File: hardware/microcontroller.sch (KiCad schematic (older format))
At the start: 30 parts, among them P1 USB_OTG, P2 ICSP, P3 JTAG, SW1 Reset, U1 ATMEGA32U4-AU, X1 16MHz

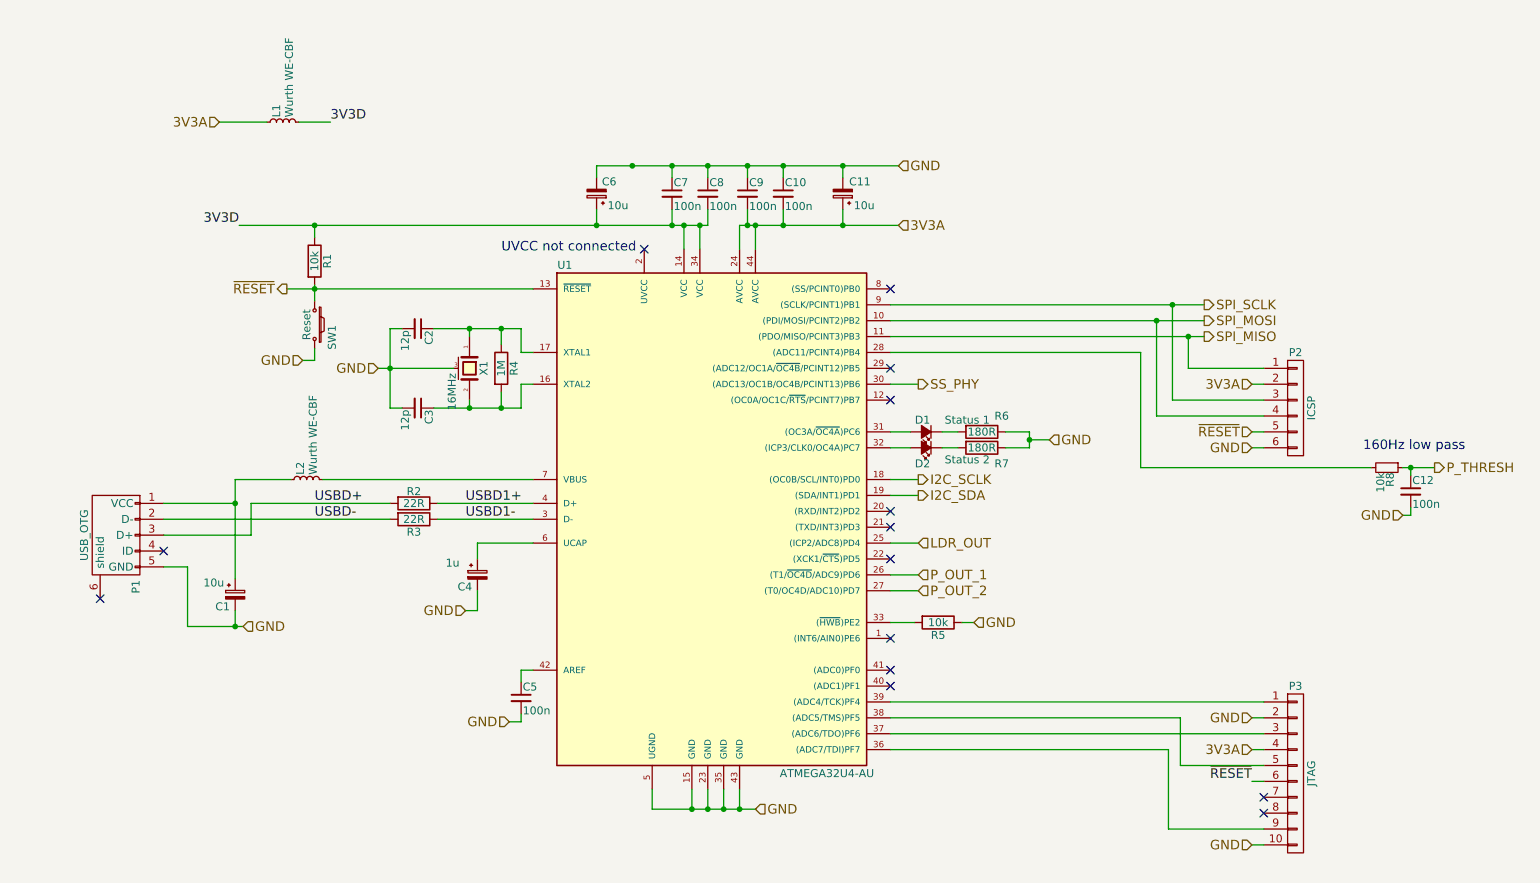
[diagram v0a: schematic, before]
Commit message: New revision to board
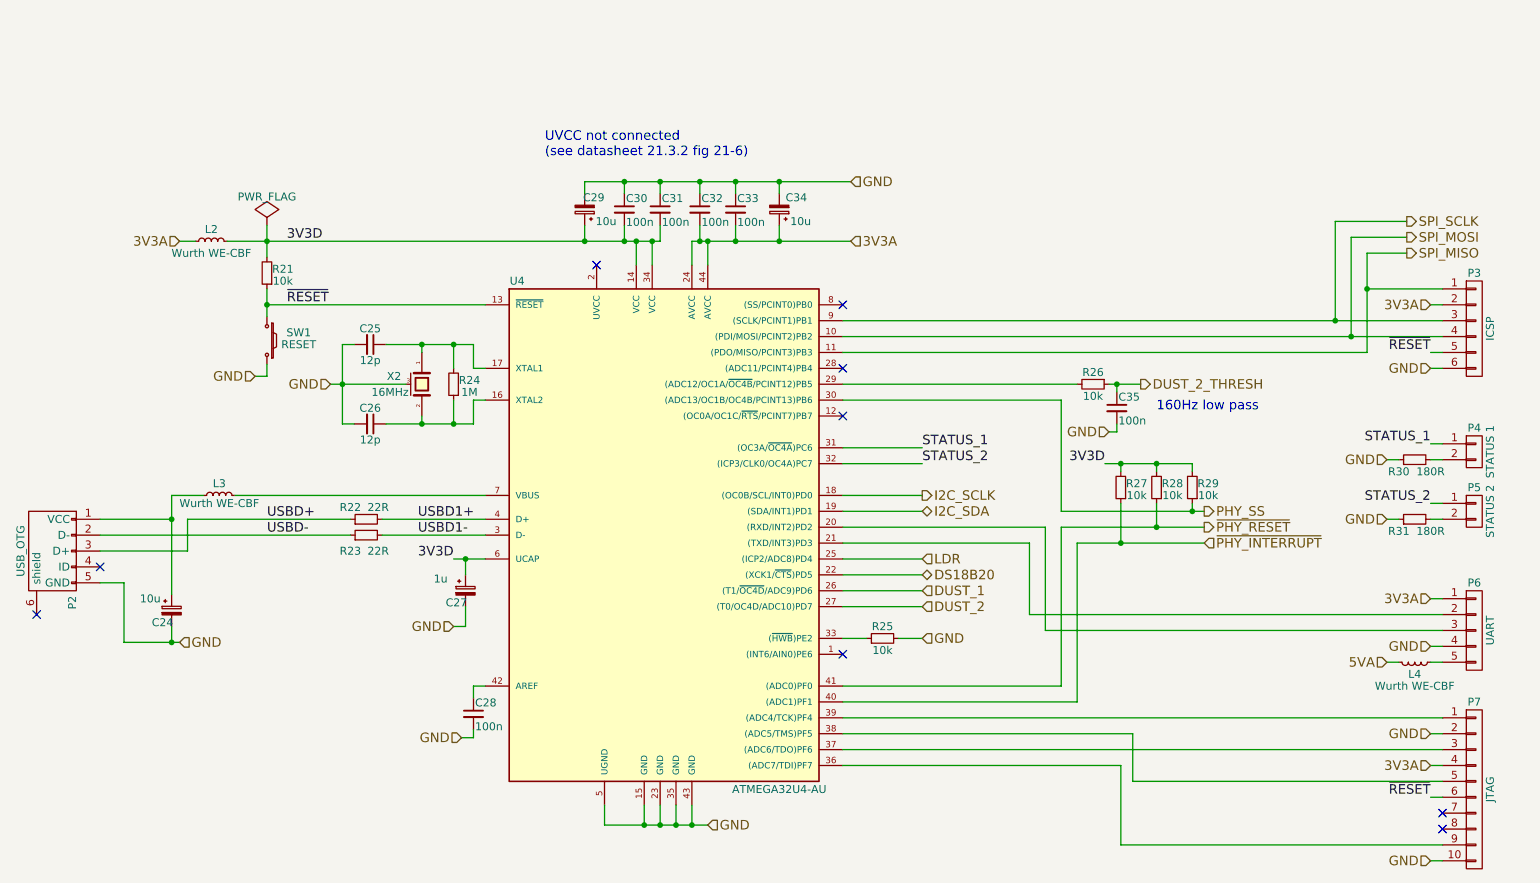
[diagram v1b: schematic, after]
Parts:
- removed C2: 12p, Capacitors_SMD:C_0603, symbol C_Small
- removed D1: Status 1, Connectors_Molex:Molex_KK-6410-02_02x2.54mm_Straight, symbol Led_Small
- removed D2: Status 2, Connectors_Molex:Molex_KK-6410-02_02x2.54mm_Straight, symbol Led_Small
- removed L1: Wurth WE-CBF, Choke_SMD:Choke_SMD_1206_Standard, symbol L_Small
- removed R1, R5: 10k, Resistors_SMD:R_1206, symbol R
- removed R2, R3: 22R, Resistors_SMD:R_1206, symbol R
- removed R4: 1M, Resistors_SMD:R_1206, symbol R
- removed R6, R7: 180R, Resistors_SMD:R_1206, symbol R
- added C25: 12p, Capacitors_SMD:C_0603, symbol C_Small
- added L3, L4: Wurth WE-CBF, Choke_SMD:Choke_SMD_1206_Standard, symbol L_Small
- added P4: STATUS 1, Connectors_Molex:Molex_KK-6410-02_02x2.54mm_Straight, symbol CONN_01X02
- added P5: STATUS 2, Connectors_Molex:Molex_KK-6410-02_02x2.54mm_Straight, symbol CONN_01X02
- added P6: UART, Pin_Headers:Pin_Header_Straight_1x05, symbol CONN_01X05
- added R21, R25, R27, R28, R29: 10k, Resistors_SMD:R_1206, symbol R_Small
- added R22, R23: 22R, Resistors_SMD:R_1206, symbol R_Small
- added R24: 1M, Resistors_SMD:R_1206, symbol R_Small
- added R30, R31: 180R, Resistors_SMD:R_1206, symbol R_Small
- SW1: value Reset -> RESET; footprint Buttons_Switches_SMD:SW_SPST_EVQP0 -> Buttons_Switches_SMD_FSM_JSM:SW_SPST_FSM_JSM; MPN1 (none) -> 4-1437565-1; Manuf1 (none) -> TE Connectivity; SKU1 (none) -> 479-1508; Vendor1 (none) -> RS
- renumbered C1 to C24, C3 to C26, C4 to C27, C5 to C28, C6 to C29, C7 to C30, C8 to C31, C9 to C32, C10 to C33, C11 to C34, C12 to C35, P1 to P2, P2 to P3, P3 to P7, R8 to R26, U1 to U4, X1 to X2
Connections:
- net 3V3A: now also L2.1, P6.1 (P1)
- net 3V3D: now also C27.1, L2.2, U4.6 (UCAP), R21.2, R27.2, R28.2, R29.2
- net GND: now also C25.2, P6.4 (P4), R25.2, R30.1, R31.1
- net USBD+: now also R22.1
- net USBD-: now also R23.1
- net USBD1+: now also R22.2
- net USBD1-: now also R23.2
- net ~RESET: now also R21.1
- net at C26.1, U4.16 (XTAL2), X2.2: now also R24.1
- net at U4.17 (XTAL1), X2.1: now also C25.1, R24.2
- net at U4.20 ((RXD/INT2)PD2): now also P6.3 (P3)
- net at U4.21 ((TXD/INT3)PD3): now also P6.2 (P2)
- net DS18B20: now reaches U4.22 ((XCK1/~CTS~)PD5)
- net at U4.28 ((ADC11/PCINT4)PB4): no longer R26.2
- net at U4.29 ((ADC12/OC1A/~OC4B~/PCINT12)PB5): now also R26.2
- net STATUS_1: now reaches U4.31 ((OC3A/~OC4A~)PC6)
- net STATUS_1: now also P4.1 (P1)
- net STATUS_2: now reaches U4.32 ((ICP3/CLK0/OC4A)PC7)
- net STATUS_2: now also P5.1 (P1)
- net at U4.33 ((~HWB~)PE2): now also R25.1
- net ~PHY_INTERRUPT: now reaches U4.40 ((ADC1)PF1)
- net ~PHY_INTERRUPT: now also R27.1
- net ~PHY_RESET: now reaches U4.41 ((ADC0)PF0)
- net ~PHY_RESET: now also R28.1
- net at U4.7 (VBUS): now also L3.2; no longer L2.2
- net at C24.1, P2.1 (VCC): now also L3.1; no longer L2.1
- net LDR_OUT renamed LDR
- net P_OUT_1 renamed DUST_1
- net P_OUT_2 renamed DUST_2
- net P_THRESH renamed DUST_2_THRESH
- net SS_PHY renamed PHY_SS
- net PHY_SS: now also R29.1
- new net: P4.2 (P2), R30.2
- new net: P5.2 (P2), R31.2
- new net: L4.1, P6.5 (P5)
- new net 5VA: L4.2
- no-connect marks 14 -> 9
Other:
- note added: "UVCC not connected\n(see datasheet 21.3.2 fig 21-6)"
- note removed: "UVCC not connected"
- moved on the sheet: C24, C26, C27, C28, C29, C30, C31, C32, C33, C34, C35, P2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
